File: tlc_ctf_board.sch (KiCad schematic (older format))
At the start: 13 parts, among them J1 AVR-ISP-6, U1 ATtiny84A-SSU

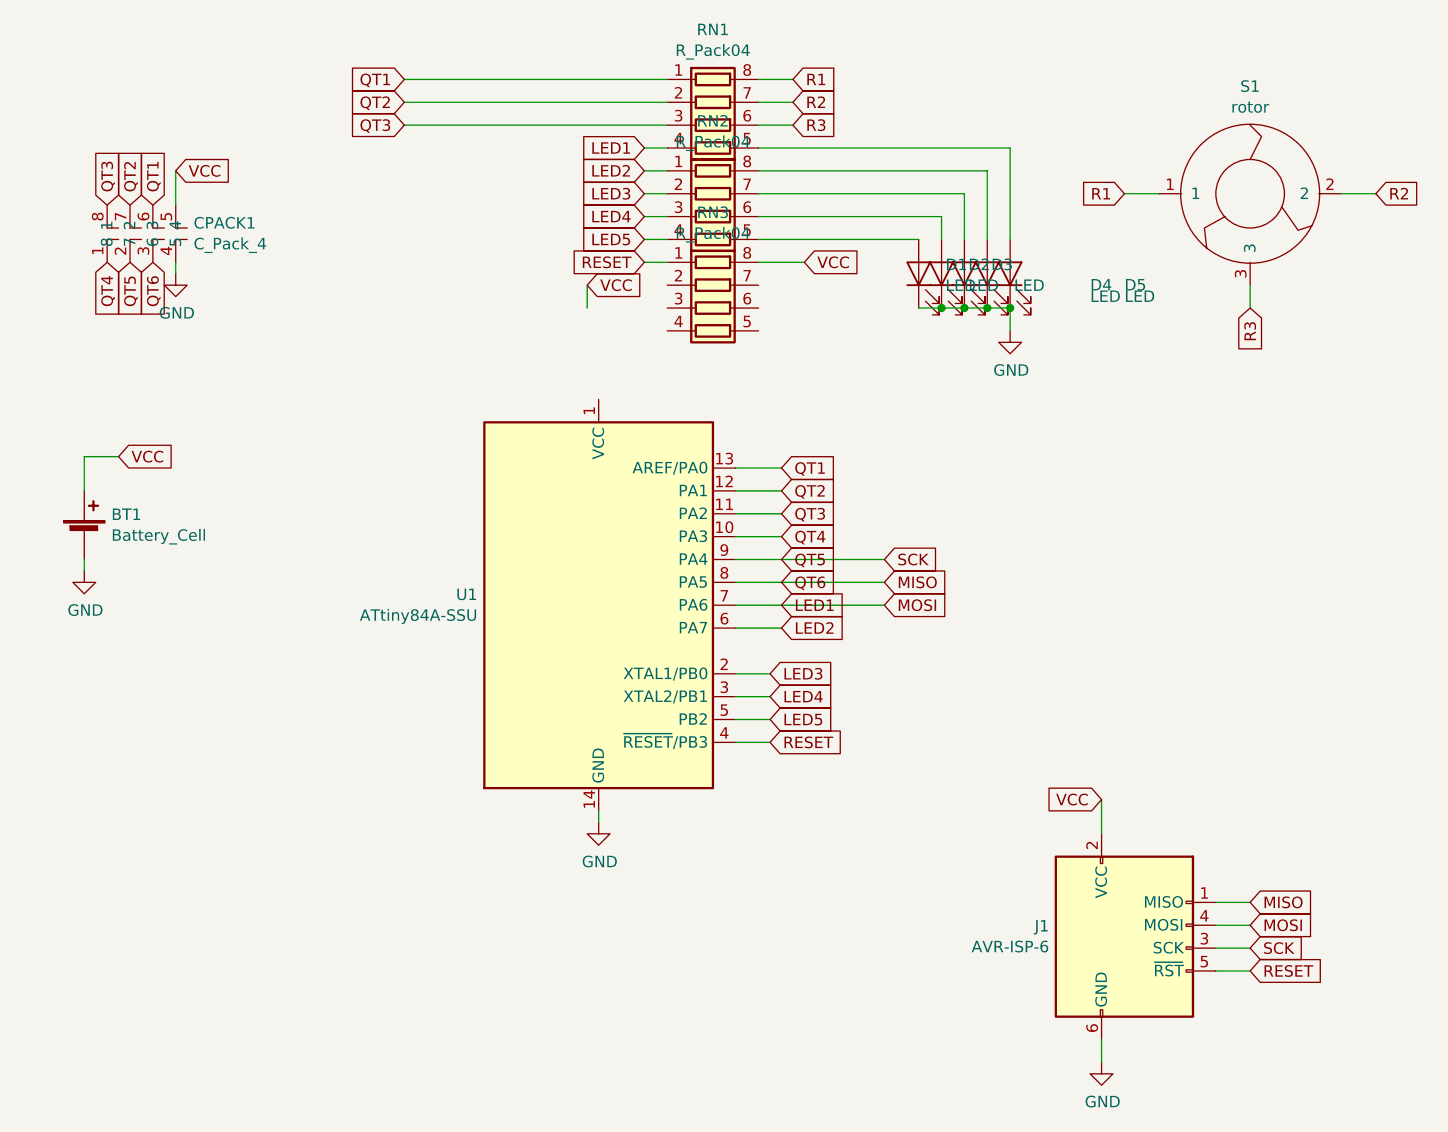
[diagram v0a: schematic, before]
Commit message: pcb mostly done
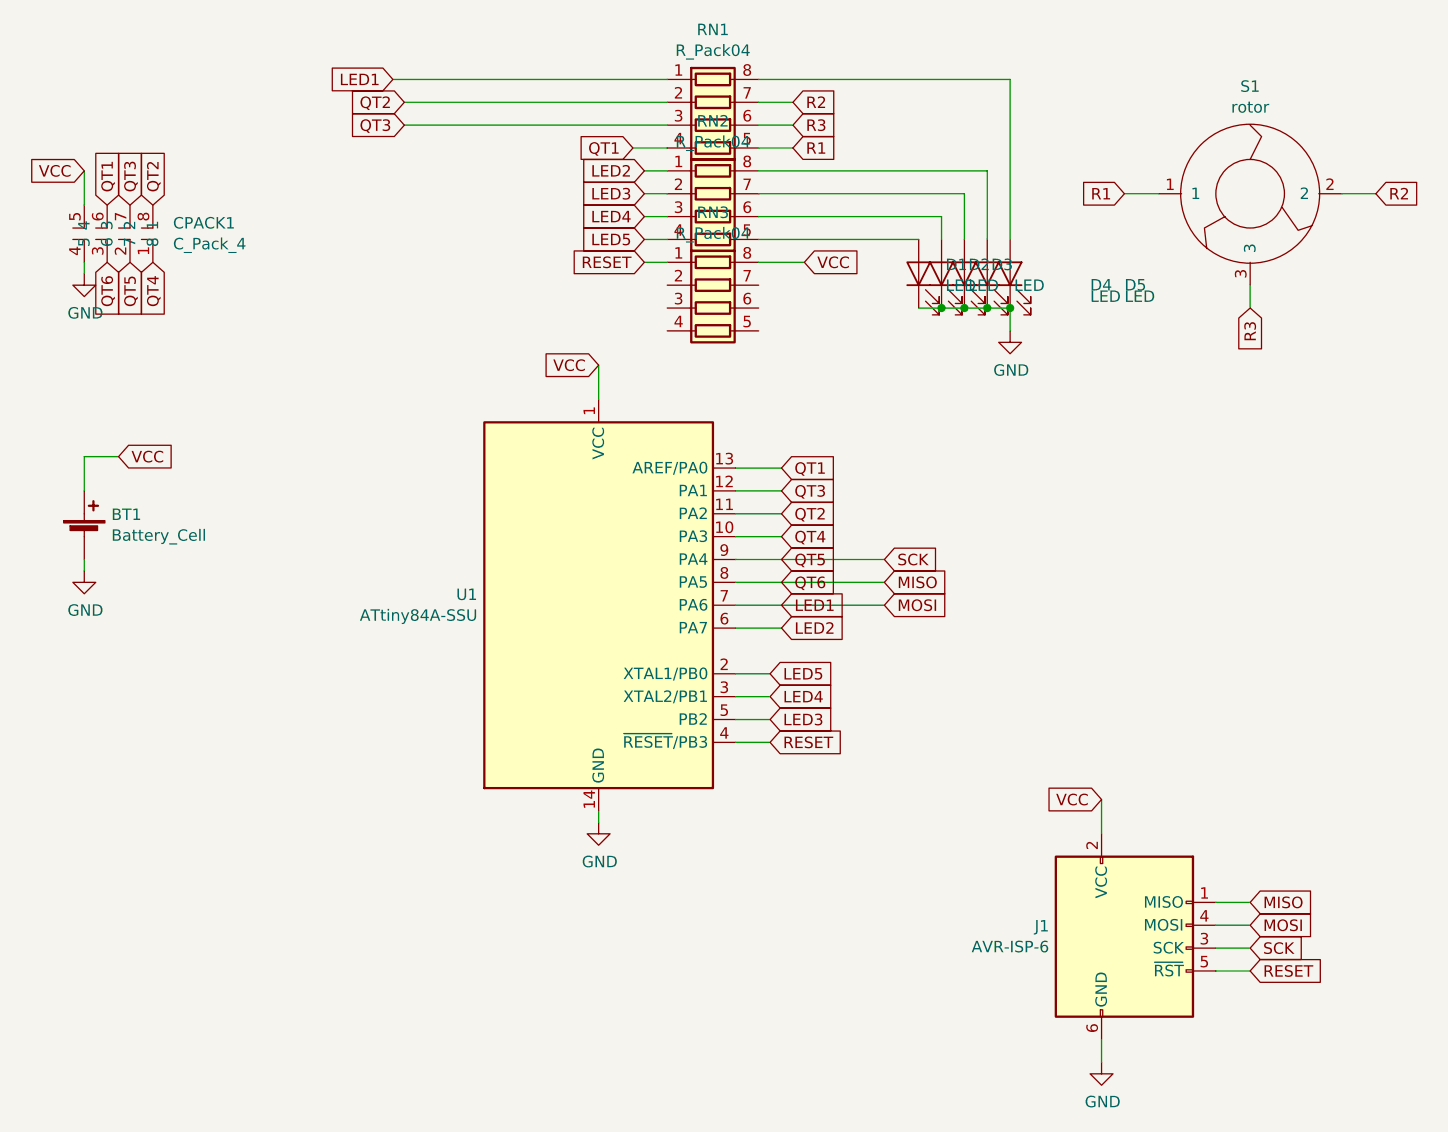
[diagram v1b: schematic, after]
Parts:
- BT1: footprint (none) -> Battery:BatteryHolder_Keystone_3034_1x20mm
- CPACK1: footprint (none) -> tlc_ctf_board:CAP_ARRAY_4_1206
- D1, D2, D3, D4, D5: footprint (none) -> digikey-footprints:LED_0603
- J1: footprint (none) -> misc_footprints:AVR-ISP-6
- RN1, RN2, RN3: footprint (none) -> tlc_ctf_board:r_array
- S1: footprint (none) -> tlc_ctf_board:wheel_simple
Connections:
- net LED1: now also RN1.1 (R1.1); no longer RN1.4 (R4.1)
- net LED3: now also U1.5 (PB2); no longer U1.2 (XTAL1/PB0)
- net LED5: now also U1.2 (XTAL1/PB0); no longer U1.5 (PB2)
- net QT1: now also RN1.4 (R4.1); no longer RN1.1 (R1.1)
- net QT2: now also CPACK1.8, U1.11 (PA2); no longer CPACK1.7, U1.12 (PA1)
- net QT3: now also CPACK1.7, U1.12 (PA1); no longer CPACK1.8, U1.11 (PA2)
- net R1: now also RN1.5 (R4.2); no longer RN1.8 (R1.2)
- net VCC: now also U1.1 (VCC)
- net at D5.2 (A): now also RN1.8 (R1.2); no longer RN1.5 (R4.2)
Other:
- moved on the sheet: CPACK1
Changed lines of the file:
@@
 F 0 "BT1" H 3168 3396 50  0000 L CNN
 F 1 "Battery_Cell" H 3168 3305 50  0000 L CNN
-F 2 "" V 3050 3360 50  0001 C CNN
+F 2 "Battery:BatteryHolder_Keystone_3034_1x20mm" V 3050 3360 50  0001 C CNN
 F 3 "~" V 3050 3360 50  0001 C CNN
 	1    3050 3300
@@
 Wire Wire Line
 	3050 2950 3050 3100
-Text GLabel 5250 2200 2    50   Input ~ 0
-VCC
-Wire Wire Line
-	5250 2200 5250 2300
 $Comp
 L tlc:rotor S1
@@
 F 0 "S1" H 8150 2269 50  0000 C CNN
 F 1 "rotor" H 8150 2178 50  0000 C CNN
-F 2 "" H 8150 1800 50  0001 C CNN
+F 2 "tlc_ctf_board:wheel_simple" H 8150 1800 50  0001 C CNN
 F 3 "" H 8150 1800 50  0001 C CNN
 	1    8150 1800
@@
 QT1
 Text GLabel 6100 3100 2    50   Input ~ 0
+QT3
+Text GLabel 6100 3200 2    50   Input ~ 0
 QT2
-Text GLabel 6100 3200 2    50   Input ~ 0
-QT3
 Text GLabel 6100 3300 2    50   Input ~ 0
 QT4
@@
 Wire Wire Line
 	5900 3300 6100 3300
-Text GLabel 6150 1300 2    50   Input ~ 0
+Text GLabel 6150 1600 2    50   Input ~ 0
 R1
 Text GLabel 6150 1400 2    50   Input ~ 0
@@
 R3
 Wire Wire Line
-	6150 1300 6000 1300
-Wire Wire Line
 	6150 1400 6000 1400
 Wire Wire Line
 	6150 1500 6000 1500
-Text GLabel 4450 1300 0    50   Input ~ 0
+Text GLabel 5450 1600 0    50   Input ~ 0
 QT1
 Text GLabel 4450 1400 0    50   Input ~ 0
@@
 QT3
 Text GLabel 3150 2100 3    50   Input ~ 0
-QT4
+QT6
 Text GLabel 3250 2100 3    50   Input ~ 0
 QT5
 Text GLabel 3350 2100 3    50   Input ~ 0
-QT6
+QT4
 Text GLabel 6100 3600 2    50   Input ~ 0
 LED1
@@
 LED2
 Text GLabel 6050 3900 2    50   Input ~ 0
-LED3
+LED5
 Text GLabel 6050 4000 2    50   Input ~ 0
 LED4
 Text GLabel 6050 4100 2    50   Input ~ 0
-LED5
+LED3
 Wire Wire Line
 	5900 3900 6050 3900
@@
 Wire Wire Line
 	5900 3700 6100 3700
-Text GLabel 5500 1600 0    50   Input ~ 0
+Text GLabel 4400 1300 0    50   Input ~ 0
 LED1
 Text GLabel 5500 1700 0    50   Input ~ 0
@@
 LED5
 Wire Wire Line
-	5500 1600 5600 1600
-Wire Wire Line
 	5500 1700 5600 1700
 Wire Wire Line
@@
 F 0 "D1" V 6739 2033 50  0000 R CNN
 F 1 "LED" V 6648 2033 50  0000 R CNN
-F 2 "" H 6700 2150 50  0001 C CNN
+F 2 "digikey-footprints:LED_0603" H 6700 2150 50  0001 C CNN
 F 3 "~" H 6700 2150 50  0001 C CNN
 	1    6700 2150
@@
 F 0 "D2" V 6839 2033 50  0000 R CNN
 F 1 "LED" V 6748 2033 50  0000 R CNN
-F 2 "" H 6800 2150 50  0001 C CNN
+F 2 "digikey-footprints:LED_0603" H 6800 2150 50  0001 C CNN
 F 3 "~" H 6800 2150 50  0001 C CNN
 	1    6800 2150
@@
 F 0 "D3" V 6939 2033 50  0000 R CNN
 F 1 "LED" V 6800 1600 50  0000 R CNN
-F 2 "" H 6900 2150 50  0001 C CNN
+F 2 "digikey-footprints:LED_0603" H 6900 2150 50  0001 C CNN
 F 3 "~" H 6900 2150 50  0001 C CNN
 	1    6900 2150
@@
 F 0 "D4" V 6950 1700 50  0000 R CNN
 F 1 "LED" V 6948 2033 50  0000 R CNN
-F 2 "" H 7000 2150 50  0001 C CNN
+F 2 "digikey-footprints:LED_0603" H 7000 2150 50  0001 C CNN
 F 3 "~" H 7000 2150 50  0001 C CNN
 	1    7000 2150
@@
 F 0 "D5" V 7050 1650 50  0000 R CNN
 F 1 "LED" V 7000 1650 50  0000 R CNN
-F 2 "" H 7100 2150 50  0001 C CNN
+F 2 "digikey-footprints:LED_0603" H 7100 2150 50  0001 C CNN
 F 3 "~" H 7100 2150 50  0001 C CNN
 	1    7100 2150
@@
 	6000 1700 7000 1700
 Wire Wire Line
-	7100 1600 7100 2000
-Wire Wire Line
-	6000 1600 7100 1600
-Wire Wire Line
 	6100 3000 5900 3000
 Text GLabel 6050 4200 2    50   Input ~ 0
@@
 F 0 "J1" H 7271 5196 50  0000 R CNN
 F 1 "AVR-ISP-6" H 7271 5105 50  0000 R CNN
-F 2 "" V 7350 5150 50  0001 C CNN
+F 2 "misc_footprints:AVR-ISP-6" V 7350 5150 50  0001 C CNN
 F 3 " ~" H 6325 4550 50  0001 C CNN
 	1    7600 5100
@@
 Wire Wire Line
 	5900 3600 6550 3600
-Text GLabel 3450 1700 2    50   Input ~ 0
-VCC
-Wire Wire Line
-	3450 1700 3450 1850
+Text GLabel 3050 1700 0    50   Input ~ 0
+VCC
 $Comp
 L power:GND #PWR02
 U 1 1 5DABE4F7
-P 3450 2150
-F 0 "#PWR02" H 3450 1900 50  0001 C CNN
-F 1 "GND" H 3455 1977 50  0000 C CNN
-F 2 "" H 3450 2150 50  0001 C CNN
-F 3 "" H 3450 2150 50  0001 C CNN
-	1    3450 2150
-	1    0    0    -1
-$EndComp
-Wire Wire Line
-	3450 2150 3450 2100
+P 3050 2150
+F 0 "#PWR02" H 3050 1900 50  0001 C CNN
+F 1 "GND" H 3055 1977 50  0000 C CNN
+F 2 "" H 3050 2150 50  0001 C CNN
+F 3 "" H 3050 2150 50  0001 C CNN
+	1    3050 2150
+	1    0    0    -1
+$EndComp
+Wire Wire Line
+	3050 2150 3050 2100
 $Comp
 L Device:R_Pack04 RN1
@@
 F 0 "RN1" V 5383 1500 50  0000 C CNN
 F 1 "R_Pack04" V 5474 1500 50  0000 C CNN
-F 2 "" V 6075 1500 50  0001 C CNN
+F 2 "tlc_ctf_board:r_array" V 6075 1500 50  0001 C CNN
 F 3 "~" H 5800 1500 50  0001 C CNN
 	1    5800 1500
@@
 F 0 "RN2" V 5383 1900 50  0000 C CNN
 F 1 "R_Pack04" V 5474 1900 50  0000 C CNN
-F 2 "" V 6075 1900 50  0001 C CNN
+F 2 "tlc_ctf_board:r_array" V 6075 1900 50  0001 C CNN
 F 3 "~" H 5800 1900 50  0001 C CNN
 	1    5800 1900
@@
 F 0 "RN3" V 5383 2300 50  0000 C CNN
 F 1 "R_Pack04" V 5474 2300 50  0000 C CNN
-F 2 "" V 6075 2300 50  0001 C CNN
+F 2 "tlc_ctf_board:r_array" V 6075 2300 50  0001 C CNN
 F 3 "~" H 5800 2300 50  0001 C CNN
 	1    5800 2300
@@
 Wire Wire Line
 	4450 1400 5600 1400
-Wire Wire Line
-	4450 1300 5600 1300
+Text GLabel 3350 1850 1    50   Input ~ 0
+QT2
+Text GLabel 3250 1850 1    50   Input ~ 0
+QT3
+Text GLabel 3150 1850 1    50   Input ~ 0
+QT1
+Wire Wire Line
+	6700 2300 6800 2300
+Connection ~ 6800 2300
+Wire Wire Line
+	6800 2300 6900 2300
+Connection ~ 6900 2300
+Wire Wire Line
+	6900 2300 7000 2300
+Connection ~ 7000 2300
+Wire Wire Line
+	7000 2300 7100 2300
+Connection ~ 7100 2300
+Wire Wire Line
+	3050 1700 3050 1850
+Wire Wire Line
+	5450 1600 5600 1600
+Wire Wire Line
+	6000 1600 6150 1600
+Wire Wire Line
+	4400 1300 5600 1300
+Wire Wire Line
+	6000 1300 7100 1300
+Wire Wire Line
+	7100 1300 7100 2000
 $Comp
 L tlc:C_Pack_4 CPACK1
 U 1 1 5DA3C3DE
-P 3300 2000
-F 0 "CPACK1" H 3528 2071 50  0000 L CNN
-F 1 "C_Pack_4" H 3528 1980 50  0000 L CNN
-F 2 "" H 3300 2000 50  0001 C CNN
-F 3 "" H 3300 2000 50  0001 C CNN
-	1    3300 2000
-	1    0    0    -1
-$EndComp
-Text GLabel 3350 1850 1    50   Input ~ 0
-QT1
-Text GLabel 3250 1850 1    50   Input ~ 0
-QT2
-Text GLabel 3150 1850 1    50   Input ~ 0
-QT3
-Wire Wire Line
-	6700 2300 6800 2300
-Connection ~ 6800 2300
-Wire Wire Line
-	6800 2300 6900 2300
-Connection ~ 6900 2300
-Wire Wire Line
-	6900 2300 7000 2300
-Connection ~ 7000 2300
-Wire Wire Line
-	7000 2300 7100 2300
-Connection ~ 7100 2300
+P 3200 2000
+F 0 "CPACK1" H 2962 2071 50  0000 R CNN
+F 1 "C_Pack_4" H 2962 1980 50  0000 R CNN
+F 2 "tlc_ctf_board:CAP_ARRAY_4_1206" H 3200 2000 50  0001 C CNN
+F 3 "" H 3200 2000 50  0001 C CNN
+	1    3200 2000
+	-1   0    0    -1
+$EndComp
+Text GLabel 5300 2550 0    50   Input ~ 0
+VCC
+Wire Wire Line
+	5300 2550 5300 2700
 $EndSCHEMATC
